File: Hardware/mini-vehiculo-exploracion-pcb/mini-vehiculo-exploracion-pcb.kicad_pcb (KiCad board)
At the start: 4 copper layers, 92 x 79 mm, 83 parts, among them IC3 MAX8891EXK33_V+T, J1 CÁMARA, J3 UJ20-C-H-G-SMT-5-P16-TR, J8 SERVO, Q1 SI1467DH-T1-BE3, U2 ESP32-S3-WROOM-1, U3 LM358, U4 TPS561208DDCR

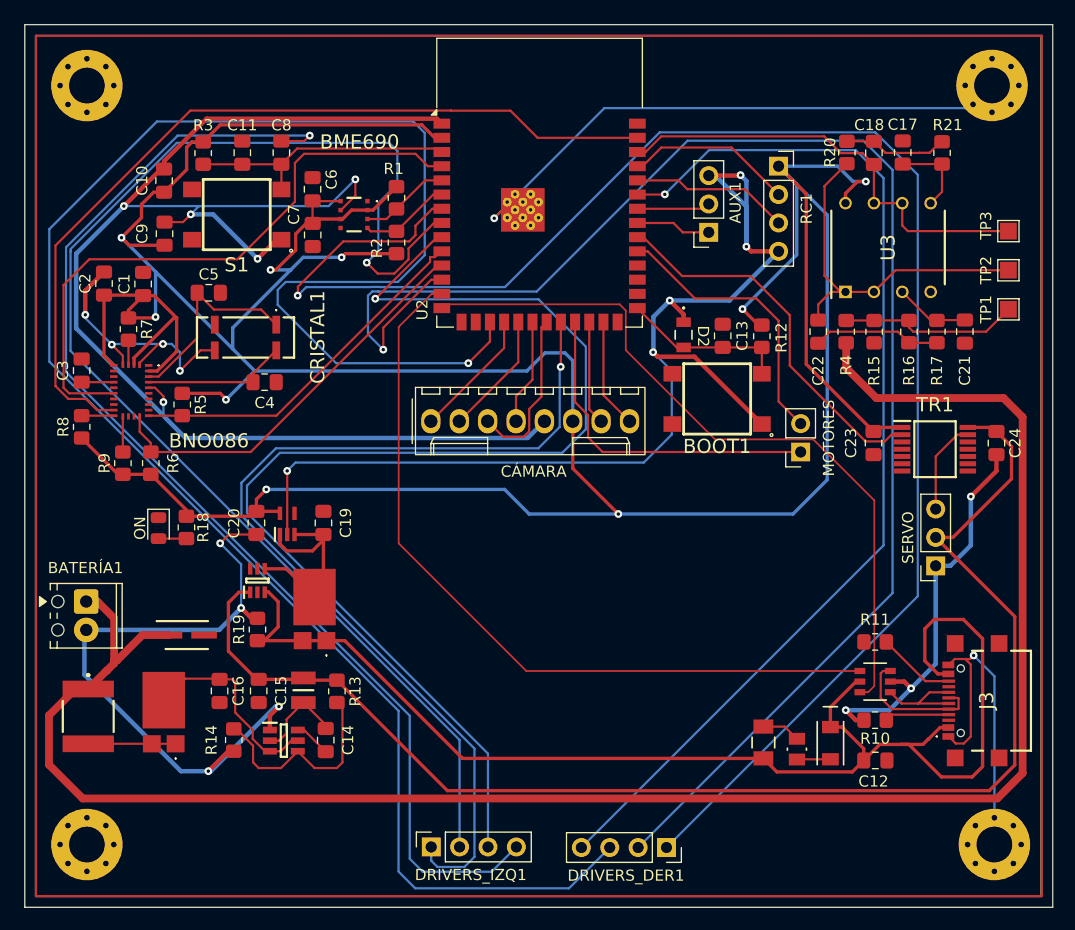
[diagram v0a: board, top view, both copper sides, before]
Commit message: update pcb4
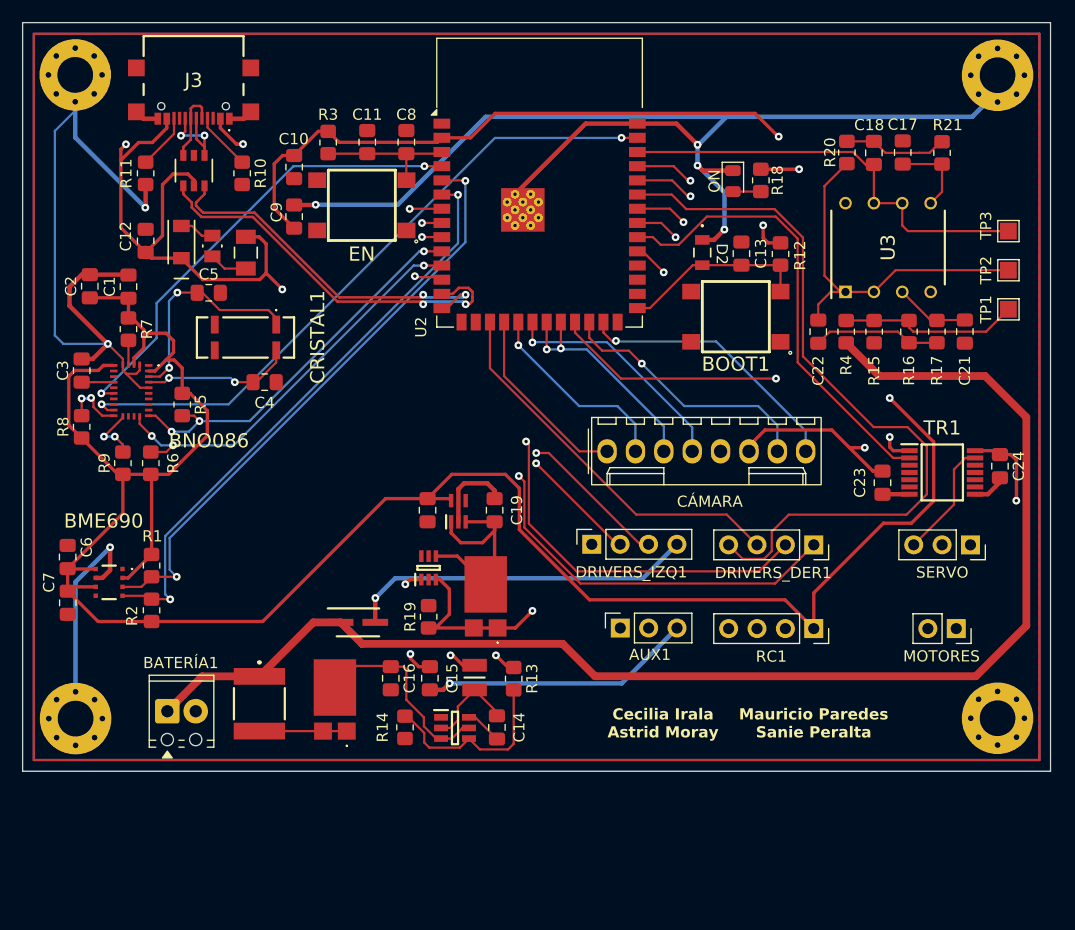
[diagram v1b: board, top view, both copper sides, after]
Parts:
- removed S1: B3FS-1010, B3FS-1010:B3FS-1000P
- added EN: B3FS-1010, B3FS-1010:B3FS-1000P, F.Cu at (115.2, 58.2)
- moved J3 90.5 mm to (100.1, 46.7), turned to 180 degrees
- moved C12 80.2 mm to (95.8, 61.4), turned to 90 degrees
- moved R11 77.6 mm to (95.8, 55.3), turned to -90 degrees
- moved CR1 76.2 mm to (100.2, 55.1), turned to -90 degrees
- moved R10 74.9 mm to (104.5, 55.3), turned to -90 degrees
- moved D1 73.4 mm to (99.0, 61.5), turned to 90 degrees
- moved FB1 69.0 mm to (101.8, 61.8), turned to 90 degrees
- moved F1 63.8 mm to (104.8, 62.4), turned to -90 degrees
- moved D6 60.1 mm to (148.4, 56.0)
- moved R18 60.1 mm to (150.9, 55.9)
- moved RC1 41.5 mm to (155.7, 96.1), turned to -90 degrees
- moved C6 39.6 mm to (88.9, 89.7)
- moved BME690 39.6 mm to (92.6, 91.9)
- moved C7 39.6 mm to (88.9, 93.7)
- moved R1 39.6 mm to (96.4, 90.4)
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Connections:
- J3 pad MP1: unconnected-(J3-PadMP1) -> GND
- J3 pad MP2: unconnected-(J3-PadMP2) -> GND
- J3 pad MP3: unconnected-(J3-PadMP3) -> GND
- J3 pad MP4: unconnected-(J3-PadMP4) -> GND
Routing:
- net GND: track 544.9 -> 267.9 mm, vias 24 -> 9
- net /M1_DISABLE: track 179.9 -> 34.6 mm, vias 1 -> 0
- net /M1_IN2: track 138.3 -> 55.7 mm, vias 1 -> 2
- net /M1_IN1: track 149.7 -> 67.5 mm, vias 1 -> 2
- net /M2_IN2: track 122.1 -> 41.1 mm, vias 1 -> 2
- net /M2_DISABLE: track 110.0 -> 41.5 mm, vias 1 -> 2
- net /M2_IN1: track 87.8 -> 21.0 mm
- net /M2_nFAULT: track 25.2 -> 71.7 mm, vias 0 -> 1
- net /SDA1: track 8.09 -> 54.0 mm, vias 0 -> 2
- net /SCL1: track 8.15 -> 53.1 mm, vias 0 -> 2
- net ENT_BAT: track 166.3 -> 121.6 mm
- net /PIN_AUX2: track 6.57 -> 43.5 mm, vias 0 -> 1
- net USB_D-: track 70.5 -> 35.2 mm, vias 0 -> 2
- net /PIN_AUX1: track 6.74 -> 42.0 mm, vias 0 -> 1
- net USB_D+: track 66.3 -> 32.5 mm, vias 0 -> 2
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- added copper zone on In2.Cu, net +3.3V
- added copper zone on In1.Cu, net GND
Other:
- board size 92 x 79 mm -> 92 x 67 mm
- board text added: "Cecilia Irala Astrid Moray"
- board text added: "Mauricio Paredes Sanie Peralta"
